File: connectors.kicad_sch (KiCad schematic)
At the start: 4 parts, among them J1 Conn_01x09_Male, J2 Conn_01x04_Male, J3 Conn_02x03_Odd_Even, J4 Conn_01x04_Male

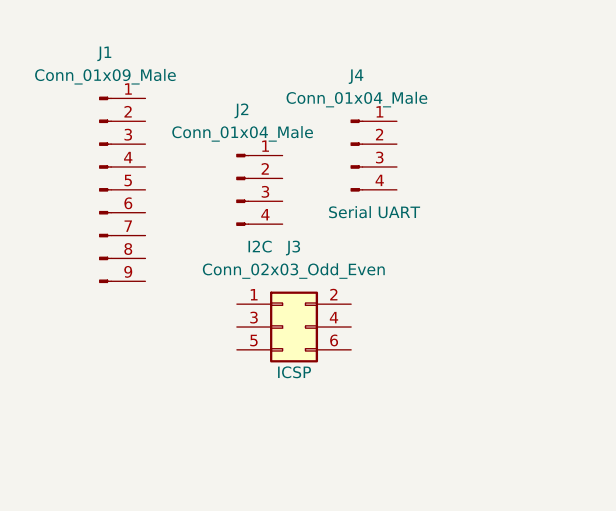
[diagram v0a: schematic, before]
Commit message: finished wiring everything up.
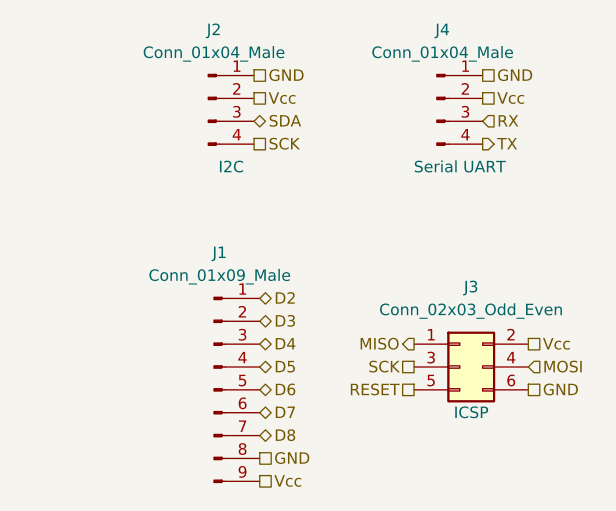
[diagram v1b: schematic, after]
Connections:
- net MISO: now reaches J3.1 (Pin_1)
- net Vcc: now reaches J3.2 (Pin_2)
- net Vcc: now also J1.9 (Pin_9), J2.2 (Pin_2), J4.2 (Pin_2)
- net SCK: now reaches J3.3 (Pin_3)
- net SCK: now also J2.4 (Pin_4)
- net MOSI: now reaches J3.4 (Pin_4)
- net RESET: now reaches J3.5 (Pin_5)
- net GND: now reaches J3.6 (Pin_6)
- net GND: now also J1.8 (Pin_8), J2.1 (Pin_1), J4.1 (Pin_1)
- net SDA: now reaches J2.3 (Pin_3)
- net D2: now reaches J1.1 (Pin_1)
- net D3: now reaches J1.2 (Pin_2)
- net D4: now reaches J1.3 (Pin_3)
- net D5: now reaches J1.4 (Pin_4)
- net D6: now reaches J1.5 (Pin_5)
- net D7: now reaches J1.6 (Pin_6)
- net D8: now reaches J1.7 (Pin_7)
- net RX: now reaches J4.3 (Pin_3)
- net TX: now reaches J4.4 (Pin_4)
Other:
- moved on the sheet: J1, J2, J3, J4
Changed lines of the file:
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@@
 (kicad_sch (version 20211123) (generator eeschema)
   (paper "A4")
-  (symbol (lib_id "Connector_Generic:Conn_02x03_Odd_Even") (at 60.96 60.96 0) (unit 1)
+  (hierarchical_label "SCK" (shape passive) (at 57.785 40.64 0)
+    (effects (font (size 1.27 1.27)) (justify left))
+  )
+  (hierarchical_label "D8" (shape bidirectional) (at 58.42 73.025 0)
+    (effects (font (size 1.27 1.27)) (justify left))
+  )
+  (hierarchical_label "Vcc" (shape passive) (at 88.265 62.865 0)
+    (effects (font (size 1.27 1.27)) (justify left))
+  )
+  (hierarchical_label "D5" (shape bidirectional) (at 58.42 65.405 0)
+    (effects (font (size 1.27 1.27)) (justify left))
+  )
+  (hierarchical_label "SDA" (shape bidirectional) (at 57.785 38.1 0)
+    (effects (font (size 1.27 1.27)) (justify left))
+  )
+  (hierarchical_label "Vcc" (shape passive) (at 83.185 35.56 0)
+    (effects (font (size 1.27 1.27)) (justify left))
+  )
+  (hierarchical_label "D6" (shape bidirectional) (at 58.42 67.945 0)
+    (effects (font (size 1.27 1.27)) (justify left))
+  )
+  (hierarchical_label "D2" (shape bidirectional) (at 58.42 57.785 0)
+    (effects (font (size 1.27 1.27)) (justify left))
+  )
+  (hierarchical_label "D7" (shape bidirectional) (at 58.42 70.485 0)
+    (effects (font (size 1.27 1.27)) (justify left))
+  )
+  (hierarchical_label "TX" (shape output) (at 83.185 40.64 0)
+    (effects (font (size 1.27 1.27)) (justify left))
+  )
+  (hierarchical_label "GND" (shape passive) (at 58.42 75.565 0)
+    (effects (font (size 1.27 1.27)) (justify left))
+  )
+  (hierarchical_label "RX" (shape input) (at 83.185 38.1 0)
+    (effects (font (size 1.27 1.27)) (justify left))
+  )
+  (hierarchical_label "D3" (shape bidirectional) (at 58.42 60.325 0)
+    (effects (font (size 1.27 1.27)) (justify left))
+  )
+  (hierarchical_label "MOSI" (shape input) (at 88.265 65.405 0)
+    (effects (font (size 1.27 1.27)) (justify left))
+  )
+  (hierarchical_label "RESET" (shape passive) (at 75.565 67.945 180)
+    (effects (font (size 1.27 1.27)) (justify right))
+  )
+  (hierarchical_label "GND" (shape passive) (at 88.265 67.945 0)
+    (effects (font (size 1.27 1.27)) (justify left))
+  )
+  (hierarchical_label "Vcc" (shape passive) (at 58.42 78.105 0)
+    (effects (font (size 1.27 1.27)) (justify left))
+  )
+  (hierarchical_label "MISO" (shape output) (at 75.565 62.865 180)
+    (effects (font (size 1.27 1.27)) (justify right))
+  )
+  (hierarchical_label "GND" (shape passive) (at 83.185 33.02 0)
+    (effects (font (size 1.27 1.27)) (justify left))
+  )
+  (hierarchical_label "SCK" (shape passive) (at 75.565 65.405 180)
+    (effects (font (size 1.27 1.27)) (justify right))
+  )
+  (hierarchical_label "D4" (shape bidirectional) (at 58.42 62.865 0)
+    (effects (font (size 1.27 1.27)) (justify left))
+  )
+  (hierarchical_label "Vcc" (shape passive) (at 57.785 35.56 0)
+    (effects (font (size 1.27 1.27)) (justify left))
+  )
+  (hierarchical_label "GND" (shape passive) (at 57.785 33.02 0)
+    (effects (font (size 1.27 1.27)) (justify left))
+  )
+  (symbol (lib_id "Connector_Generic:Conn_02x03_Odd_Even") (at 80.645 65.405 0) (unit 1)
     (in_bom yes) (on_board yes)
-    (property "Reference" "J3" (id 0) (at 62.23 52.07 0))
-    (property "Value" "Conn_02x03_Odd_Even" (id 1) (at 62.23 54.61 0))
-    (property "Footprint" "Connector_PinHeader_2.54mm:PinHeader_2x03_P2.54mm_Vertical" (id 2) (at 60.96 60.96 0)
+    (property "Reference" "J3" (id 0) (at 81.915 56.515 0))
+    (property "Value" "Conn_02x03_Odd_Even" (id 1) (at 81.915 59.055 0))
+    (property "Footprint" "Connector_PinHeader_2.54mm:PinHeader_2x03_P2.54mm_Vertical" (id 2) (at 80.645 65.405 0)
       (effects (font (size 1.27 1.27)) hide)
     )
-    (property "Datasheet" "~" (id 3) (at 60.96 60.96 0)
+    (property "Datasheet" "~" (id 3) (at 80.645 65.405 0)
       (effects (font (size 1.27 1.27)) hide)
     )
-    (property "Purpose" "ICSP" (id 4) (at 62.23 66.04 0))
+    (property "Purpose" "ICSP" (id 4) (at 81.915 70.485 0))
     (pin "1")
     (pin "2")
@@
     (pin "6")
   )
-  (symbol (lib_id "Connector:Conn_01x04_Male") (at 55.88 44.45 0) (unit 1)
+  (symbol (lib_id "Connector:Conn_01x04_Male") (at 52.705 35.56 0) (unit 1)
     (in_bom yes) (on_board yes)
-    (property "Reference" "J2" (id 0) (at 56.515 36.83 0))
-    (property "Value" "Conn_01x04_Male" (id 1) (at 56.515 39.37 0))
-    (property "Footprint" "Connector_PinHeader_2.54mm:PinHeader_1x04_P2.54mm_Vertical" (id 2) (at 55.88 44.45 0)
+    (property "Reference" "J2" (id 0) (at 53.34 27.94 0))
+    (property "Value" "Conn_01x04_Male" (id 1) (at 53.34 30.48 0))
+    (property "Footprint" "Connector_PinHeader_2.54mm:PinHeader_1x04_P2.54mm_Vertical" (id 2) (at 52.705 35.56 0)
       (effects (font (size 1.27 1.27)) hide)
     )
-    (property "Datasheet" "~" (id 3) (at 55.88 44.45 0)
+    (property "Datasheet" "~" (id 3) (at 52.705 35.56 0)
       (effects (font (size 1.27 1.27)) hide)
     )
-    (property "Purpose" "I2C" (id 4) (at 58.42 52.07 0))
+    (property "Purpose" "I2C" (id 4) (at 55.245 43.18 0))
     (pin "1")
     (pin "2")
@@
     (pin "4")
   )
-  (symbol (lib_id "Connector:Conn_01x09_Male") (at 40.64 45.72 0) (unit 1)
+  (symbol (lib_id "Connector:Conn_01x09_Male") (at 53.34 67.945 0) (unit 1)
     (in_bom yes) (on_board yes) (fields_autoplaced)
-    (property "Reference" "J1" (id 0) (at 41.275 30.48 0))
-    (property "Value" "Conn_01x09_Male" (id 1) (at 41.275 33.02 0))
-    (property "Footprint" "Connector_PinHeader_2.54mm:PinHeader_1x09_P2.54mm_Vertical" (id 2) (at 40.64 45.72 0)
+    (property "Reference" "J1" (id 0) (at 53.975 52.705 0))
+    (property "Value" "Conn_01x09_Male" (id 1) (at 53.975 55.245 0))
+    (property "Footprint" "Connector_PinHeader_2.54mm:PinHeader_1x09_P2.54mm_Vertical" (id 2) (at 53.34 67.945 0)
       (effects (font (size 1.27 1.27)) hide)
     )
-    (property "Datasheet" "~" (id 3) (at 40.64 45.72 0)
+    (property "Datasheet" "~" (id 3) (at 53.34 67.945 0)
       (effects (font (size 1.27 1.27)) hide)
     )
@@
     (pin "9")
   )
-  (symbol (lib_id "Connector:Conn_01x04_Male") (at 68.58 40.64 0) (unit 1)
+  (symbol (lib_id "Connector:Conn_01x04_Male") (at 78.105 35.56 0) (unit 1)
     (in_bom yes) (on_board yes)
-    (property "Reference" "J4" (id 0) (at 69.215 33.02 0))
-    (property "Value" "Conn_01x04_Male" (id 1) (at 69.215 35.56 0))
-    (property "Footprint" "Connector_PinHeader_2.54mm:PinHeader_1x04_P2.54mm_Vertical" (id 2) (at 68.58 40.64 0)
+    (property "Reference" "J4" (id 0) (at 78.74 27.94 0))
+    (property "Value" "Conn_01x04_Male" (id 1) (at 78.74 30.48 0))
+    (property "Footprint" "Connector_PinHeader_2.54mm:PinHeader_1x04_P2.54mm_Vertical" (id 2) (at 78.105 35.56 0)
       (effects (font (size 1.27 1.27)) hide)
     )
-    (property "Datasheet" "~" (id 3) (at 68.58 40.64 0)
+    (property "Datasheet" "~" (id 3) (at 78.105 35.56 0)
       (effects (font (size 1.27 1.27)) hide)
     )
-    (property "Purpose" "Serial UART" (id 4) (at 71.12 48.26 0))
+    (property "Purpose" "Serial UART" (id 4) (at 80.645 43.18 0))
     (pin "1")
     (pin "2")
